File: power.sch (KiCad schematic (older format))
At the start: 24 parts, among them U10 LM1117-3.3, U16 R-78E5.0-1.0, U3 STMPS2151, U7 LM1117-3.3

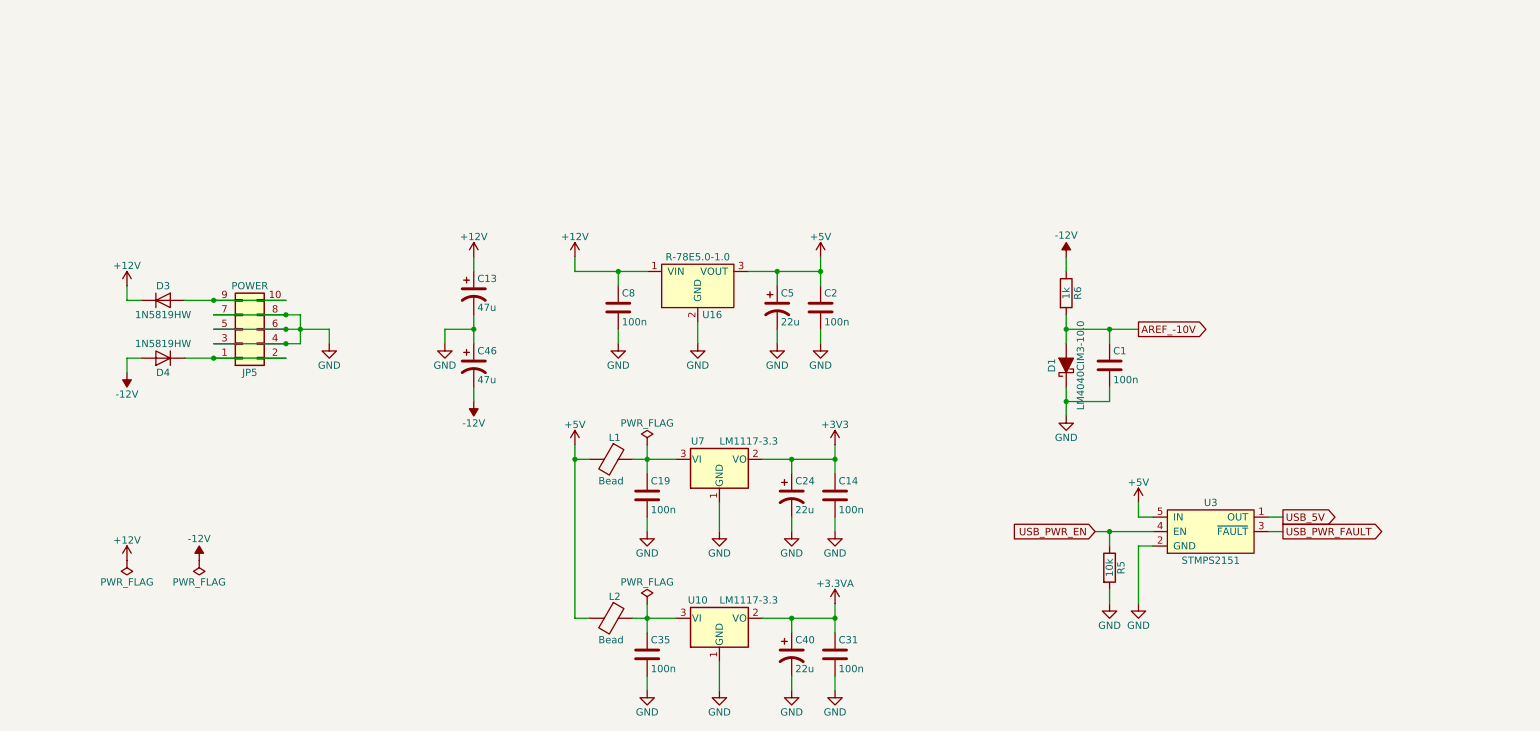
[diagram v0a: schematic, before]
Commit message: cleaned up schematics
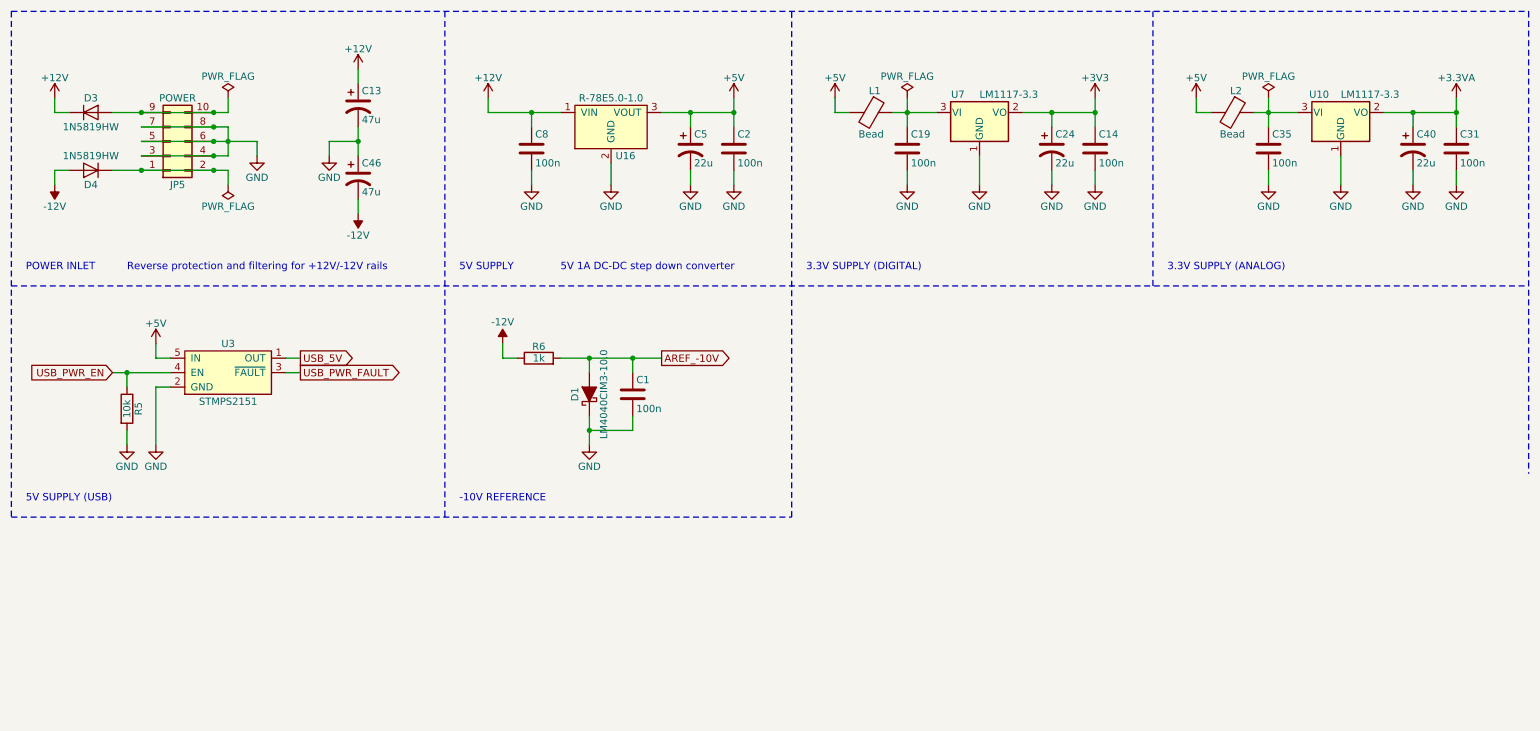
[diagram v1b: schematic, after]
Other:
- note added: "-10V REFERENCE"
- note added: "3.3V SUPPLY (ANALOG)"
- note added: "3.3V SUPPLY (DIGITAL)"
- note added: "5V 1A DC-DC step down converter"
- note added: "5V SUPPLY"
- note added: "5V SUPPLY (USB)"
- note added: "POWER INLET"
- note added: "Reverse protection and filtering for +12V/-12V rails"
- moved on the sheet: C1, C13, C14, C19, C2, C24, C31, C35, C40, C46, C5, C8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
